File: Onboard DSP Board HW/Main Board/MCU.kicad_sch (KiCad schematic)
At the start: 21 parts, among them U7 STM32H725RGVx, Y1 24Mhz

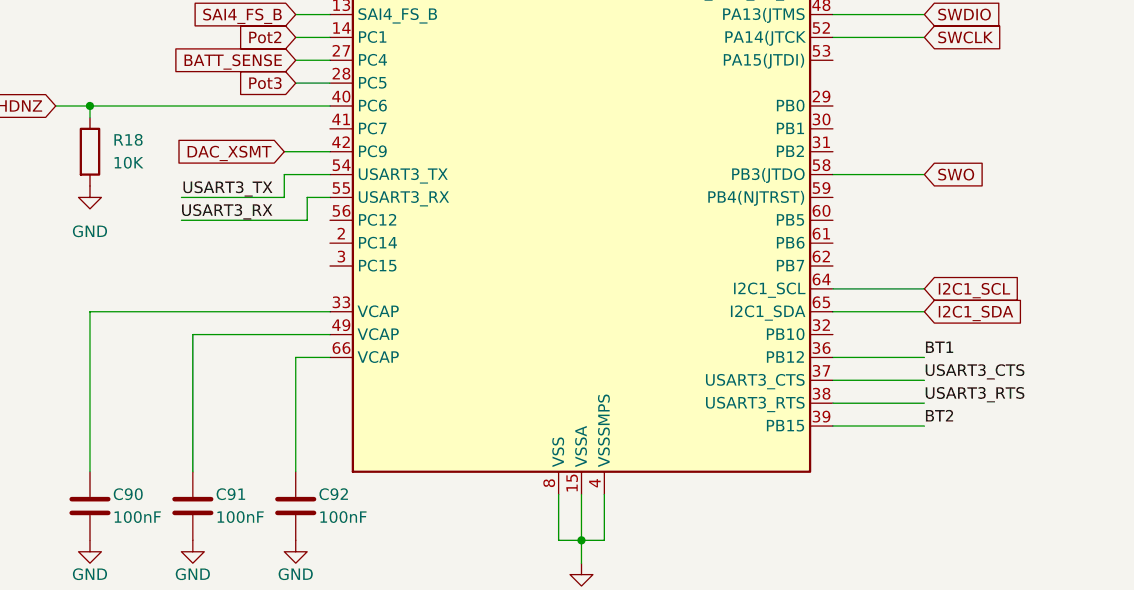
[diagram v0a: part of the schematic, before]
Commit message: WIP
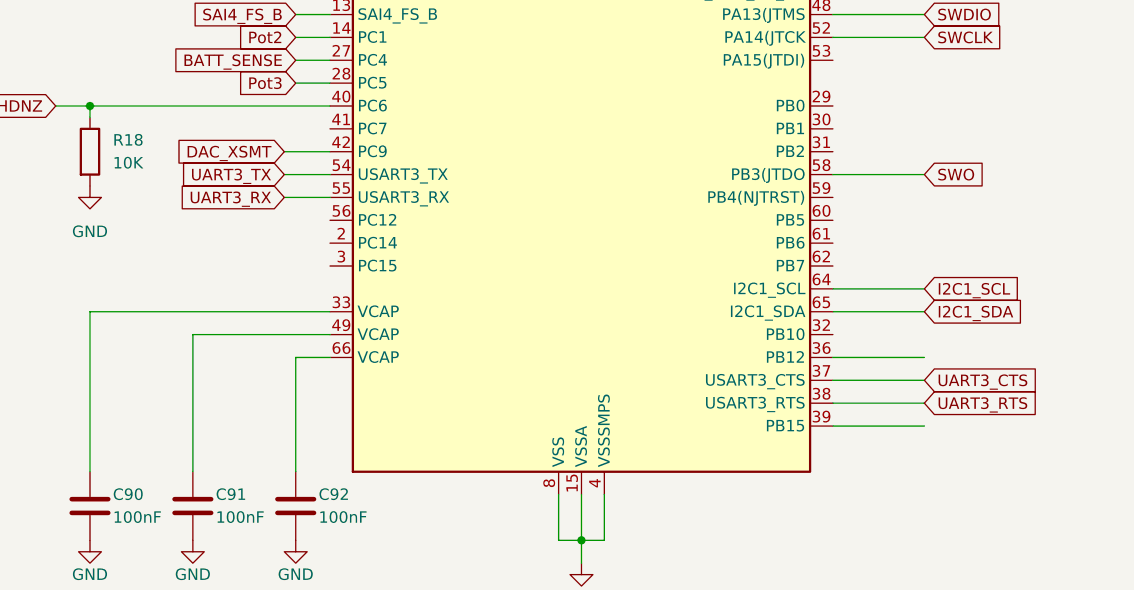
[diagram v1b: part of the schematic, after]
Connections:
- net BT1: no longer names the net of U7.36 (PB12)
- net BT2: no longer names the net of U7.39 (PB15)
- net USART3_CTS renamed UART3_CTS
- net USART3_RTS renamed UART3_RTS
- net USART3_RX renamed UART3_RX
- net USART3_TX renamed UART3_TX

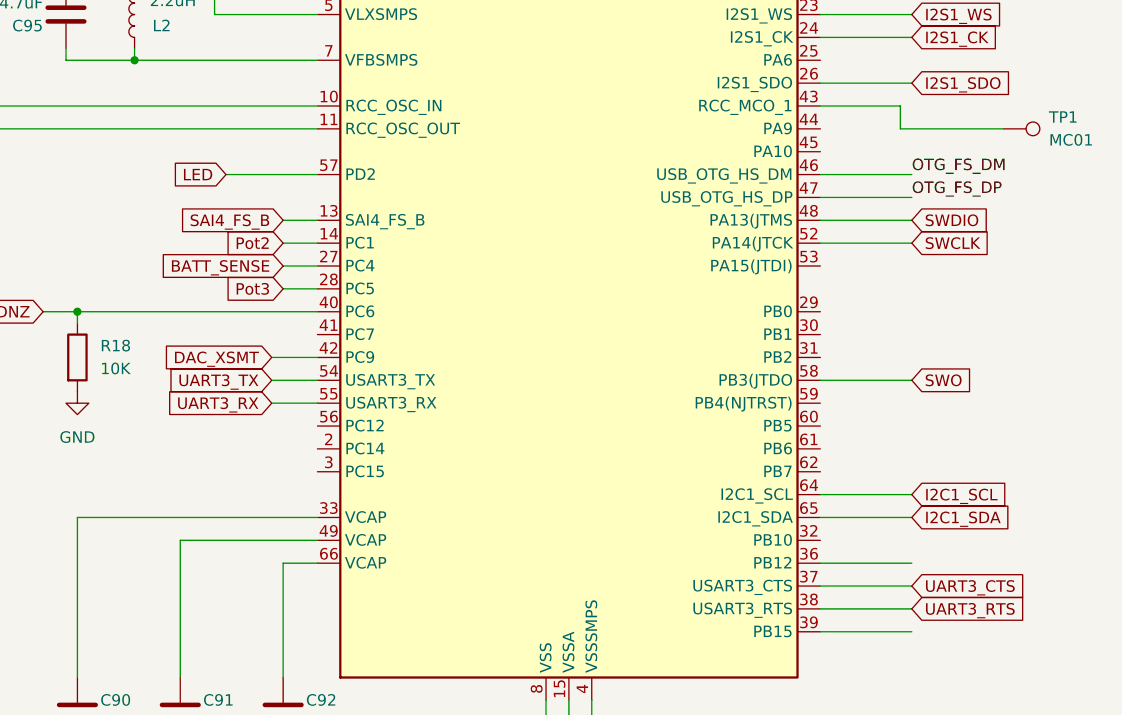
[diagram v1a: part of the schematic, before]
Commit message: WIP
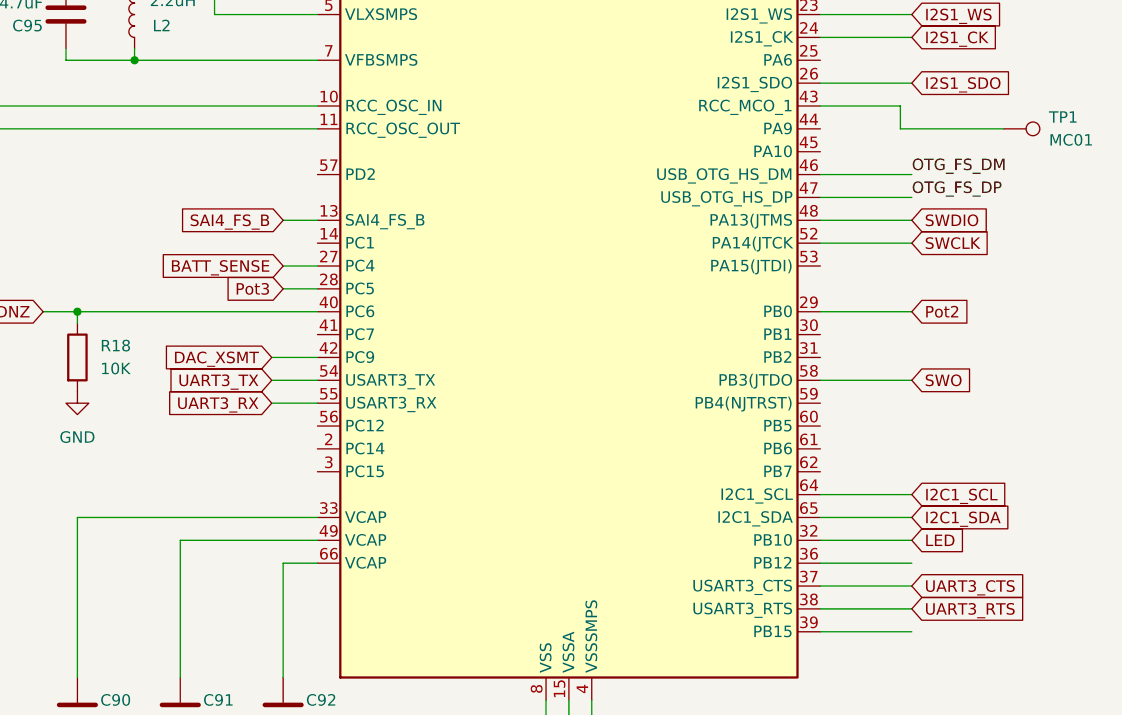
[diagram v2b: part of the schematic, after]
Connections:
- net LED: now also U7.32 (PB10); no longer U7.57 (PD2)
- net Pot2: now also U7.29 (PB0); no longer U7.14 (PC1)

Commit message: WIP
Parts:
- TP1: footprint (none) -> AWV:TestPoint_Plated_Hole_ID4_OD7.0mm
